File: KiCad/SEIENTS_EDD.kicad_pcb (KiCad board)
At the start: 2 copper layers, 147.1 x 122.2 mm, 95 parts, among them IC1 A3144EUA, J1 Conn_01x02_Pin, J201 Screw_Terminal_01x04, J3 Screw_Terminal_01x05, J4 Screw_Terminal_01x02, J7 DE9_Socket, J8 DE9_Pins, M4 Motor_DC, M5 Motor_DC, M6 Motor_DC, Q201 IRLZ44N, SW10 SW_Push, SW11 SW_Push, SW12 SW_Push, SW13 SW_Push, SW14 SW_Push, SW15 SW_Push, SW8 SW_Push, SW9 SW_Push, U1 LM2596S-5, U11 MAX3232, U2 LM1117DT-3.3, U3 MCP2562-E-SN, U4 TMP102xxDRL, U5 TB6612FNG, U6 24LC256, U67 PIC24HJ64GP504-I/PT, U7 ATtiny1616-M, U8 DRV8871DDA, Y1 8 MHz

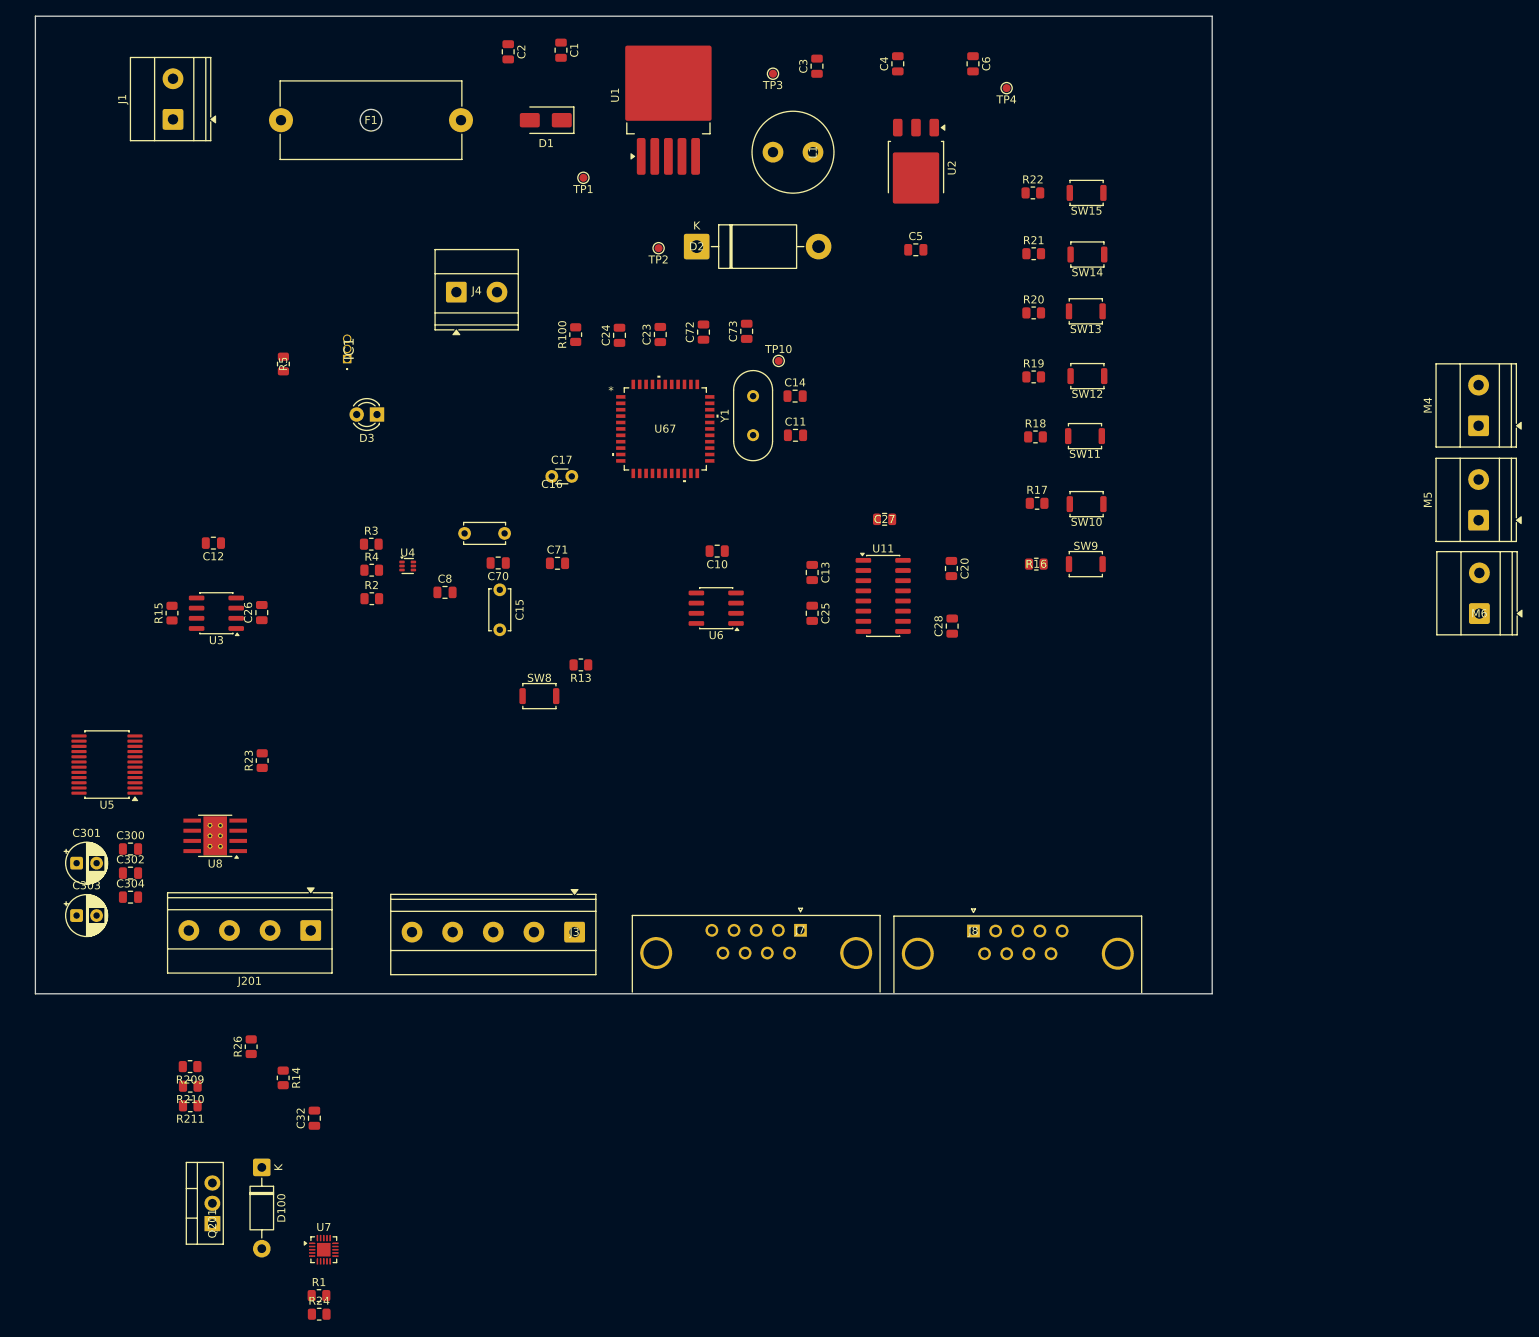
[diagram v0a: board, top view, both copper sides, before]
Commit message: Modificació al placement
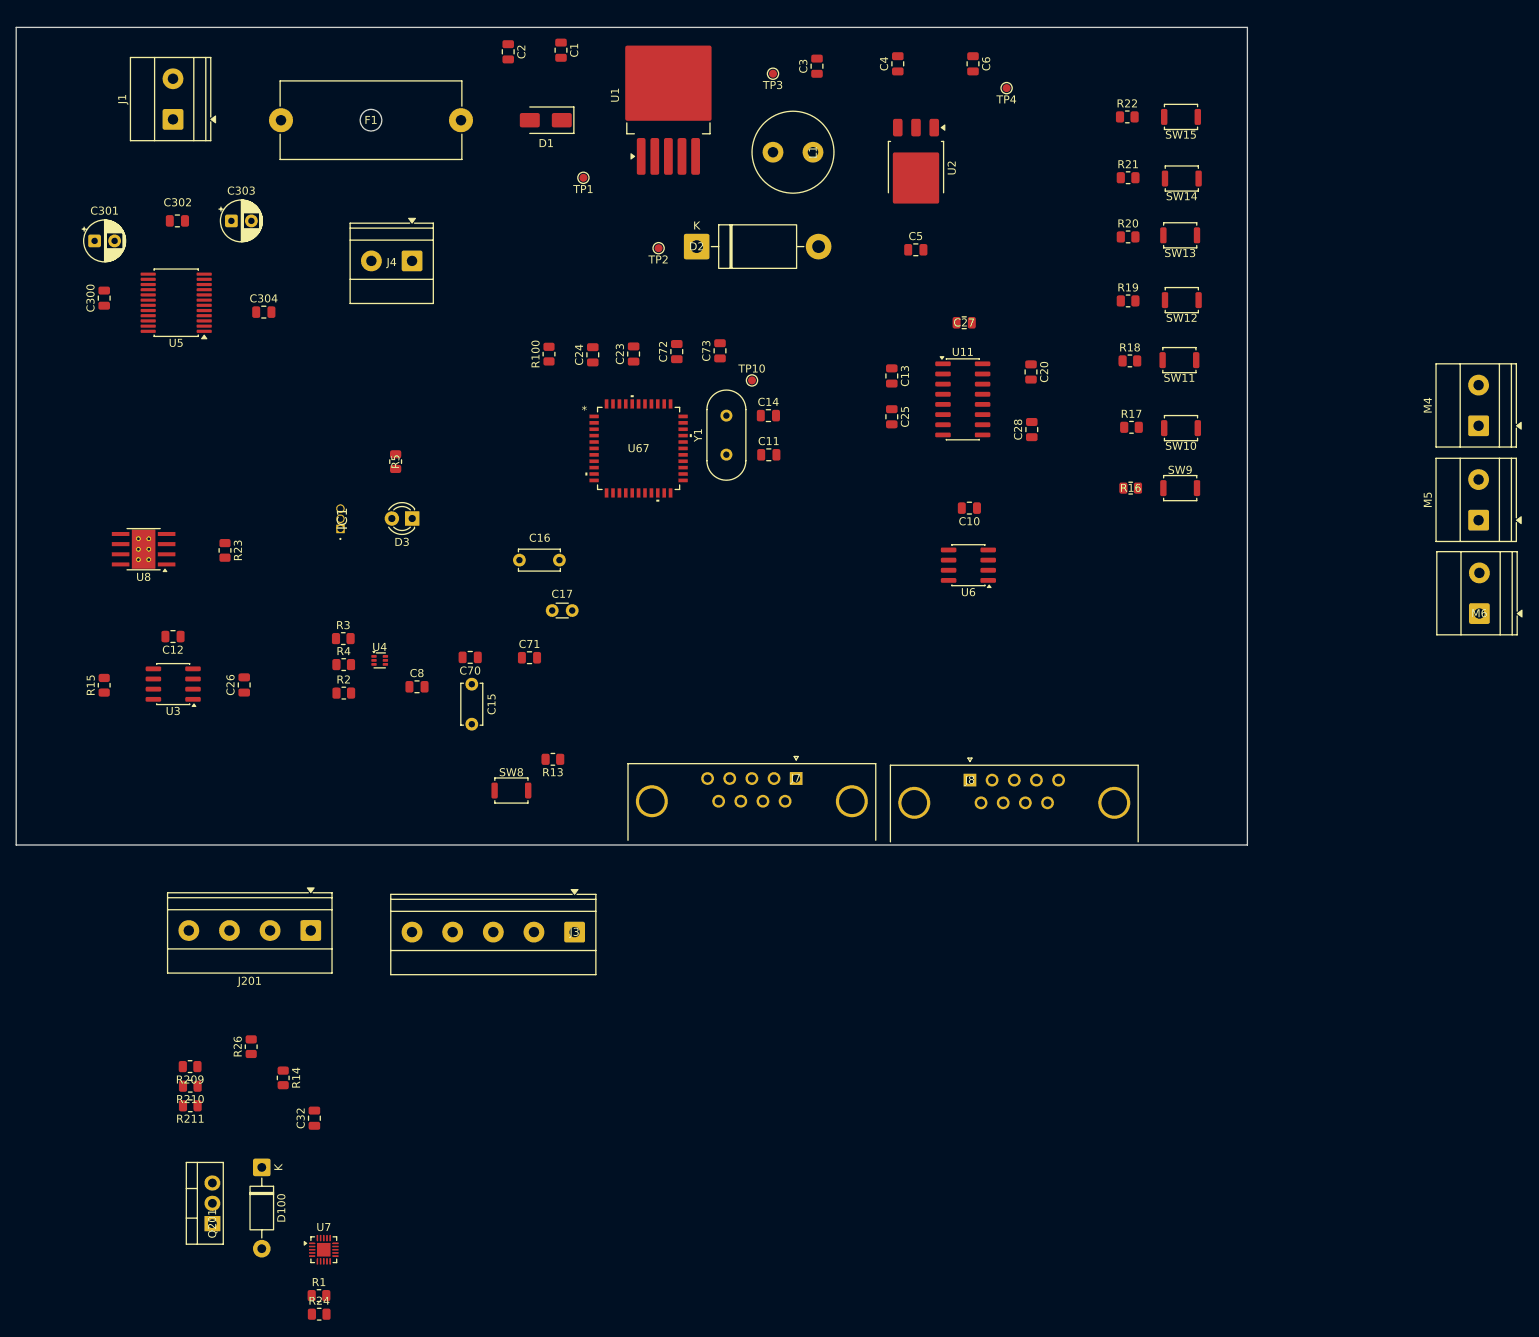
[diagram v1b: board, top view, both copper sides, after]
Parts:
- moved C303 89.0 mm to (56.4, 46.5)
- moved C302 81.7 mm to (49.6, 46.5)
- moved C301 77.8 mm to (39.3, 49.0)
- moved C304 75.0 mm to (60.5, 57.9)
- moved C300 68.9 mm to (40.5, 56.1), turned to 90 degrees
- moved U5 58.4 mm to (49.5, 56.7)
- moved U8 36.9 mm to (45.4, 87.5)
- moved C10 32.0 mm to (148.7, 82.4)
- moved U6 32.0 mm to (148.5, 89.5)
- moved R23 26.7 mm to (55.6, 87.7), turned to -90 degrees
- moved C13 26.5 mm to (138.9, 65.9)
- moved C20 26.5 mm to (156.3, 65.4)
- moved C28 26.5 mm to (156.4, 72.6)
- moved C27 26.5 mm to (148.0, 59.2)
- moved C25 26.5 mm to (138.9, 71.0)
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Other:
- board size 147.1 x 122.2 mm -> 153.9 x 102.2 mm
